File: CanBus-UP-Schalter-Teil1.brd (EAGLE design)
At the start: 42.2 x 44.3 mm, 10 parts, among them K1 36.11, K2 36.11, X1 MKDSN1,5/3-5,08, X2 MKDSN1,5/3-5,08

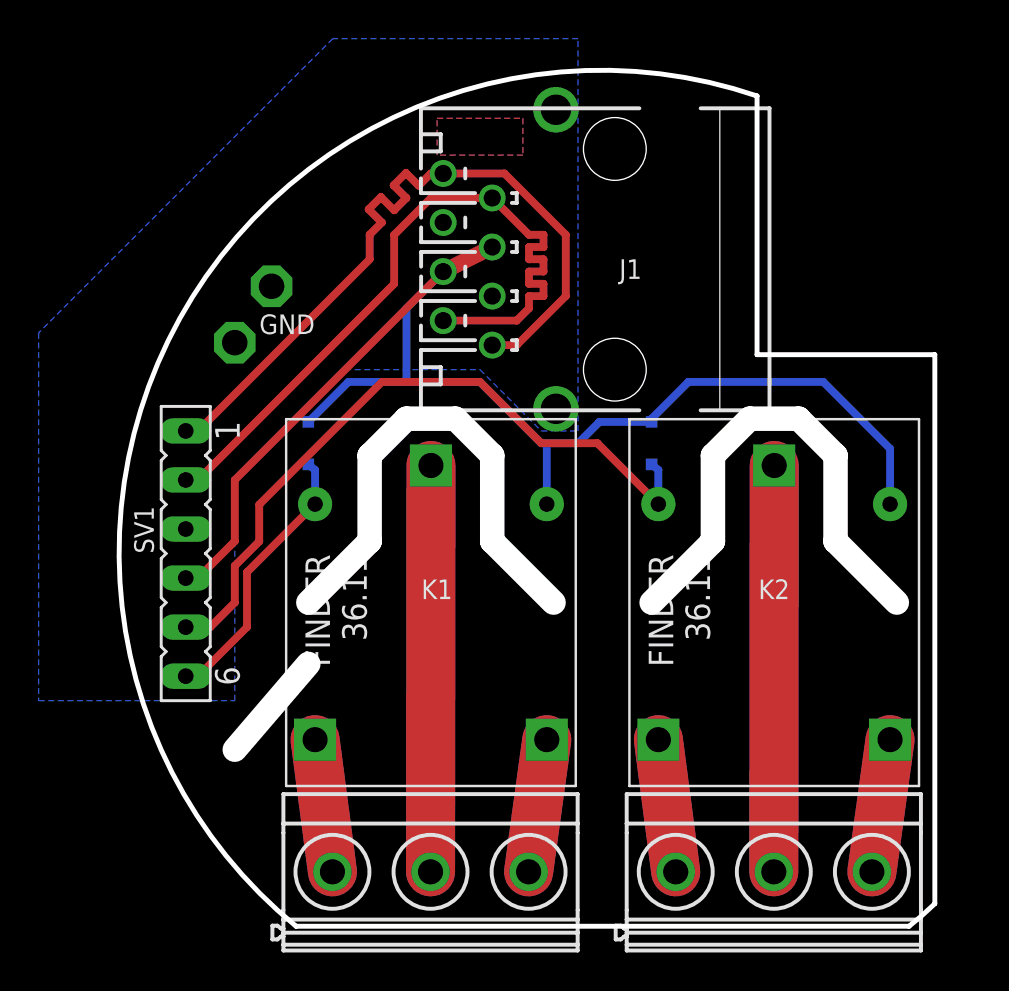
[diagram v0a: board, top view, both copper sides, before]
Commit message: CanBus-UP-Schalter fertiggestellt
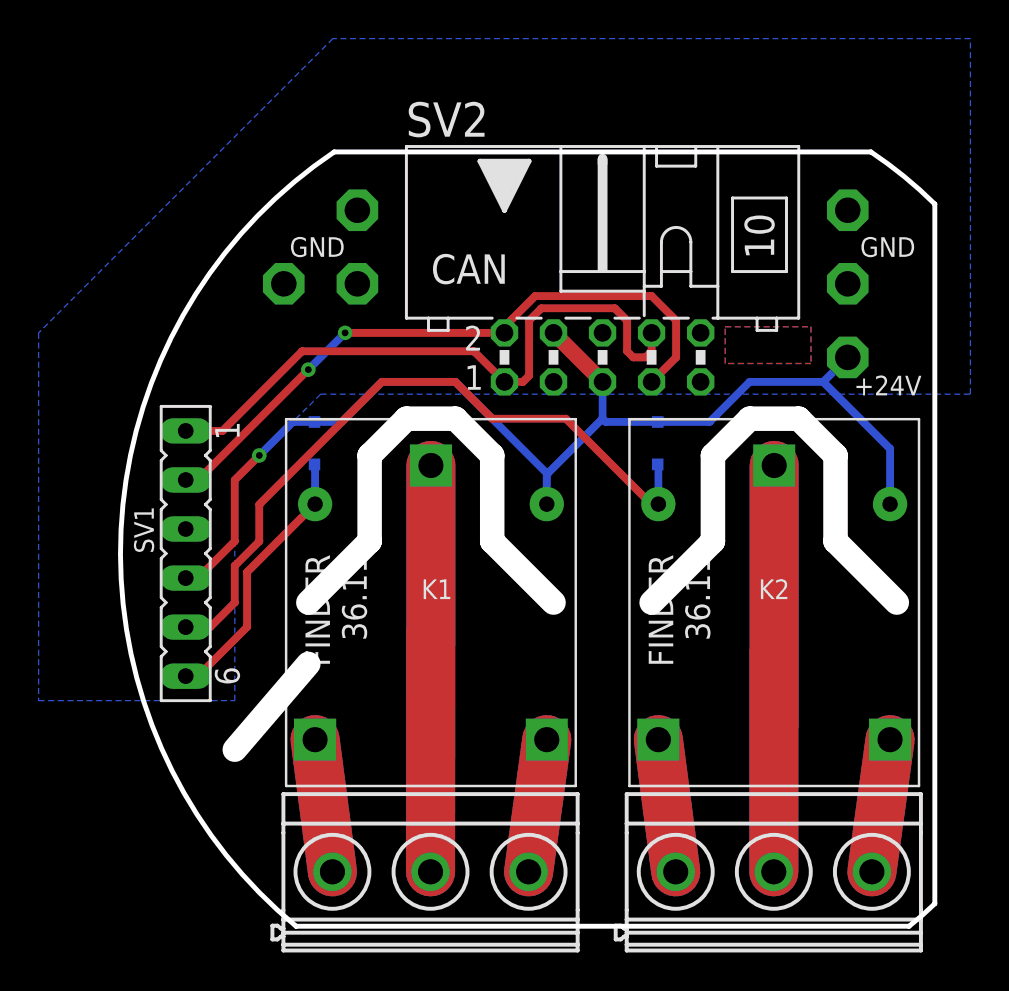
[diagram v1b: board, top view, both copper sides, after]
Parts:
- removed J1: (no value), can-bus:MEBP_8-8G
- added LSP3, LSP4, LSP5, LSP6: LSP13, solpad:LSP13
- added SV2: (no value), can-bus:ML10L
- moved LSP1 4.45 mm to (-12.7, 14.0)
- moved LSP2 3.97 mm to (-16.5, 14.0)
- moved D1 0.32 mm to (-14.9, 5.71)
- moved D2 0.32 mm to (2.86, 5.71)
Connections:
- net +24V: now also LSP6.MP, SV2.4, SV2.5; no longer J1.4, J1.5
- net CANH: now also SV2.2, SV2.7; no longer J1.2, J1.7
- net CANL: now also SV2.1, SV2.8; no longer J1.1, J1.8
- net GND: now also LSP3.MP, LSP4.MP, LSP5.MP, SV2.3, SV2.6; no longer J1.3, J1.6, J1.G1, J1.G2
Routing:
- net +24V: track 72.3 -> 59.8 mm, vias 0 -> 1
- net CANL: track 39.1 -> 32.8 mm
- net CANH: track 39.1 -> 33.8 mm, vias 0 -> 2
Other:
- board size 42.2 x 44.3 mm -> 42.2 x 40.1 mm
- board text added: "!! 230 V !!"
- board text added: "+24V"
- board text added: "L"
